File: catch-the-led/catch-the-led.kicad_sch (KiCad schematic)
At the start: 18 parts, among them SW1 SW_Push, U1 NE555P, U2 4017

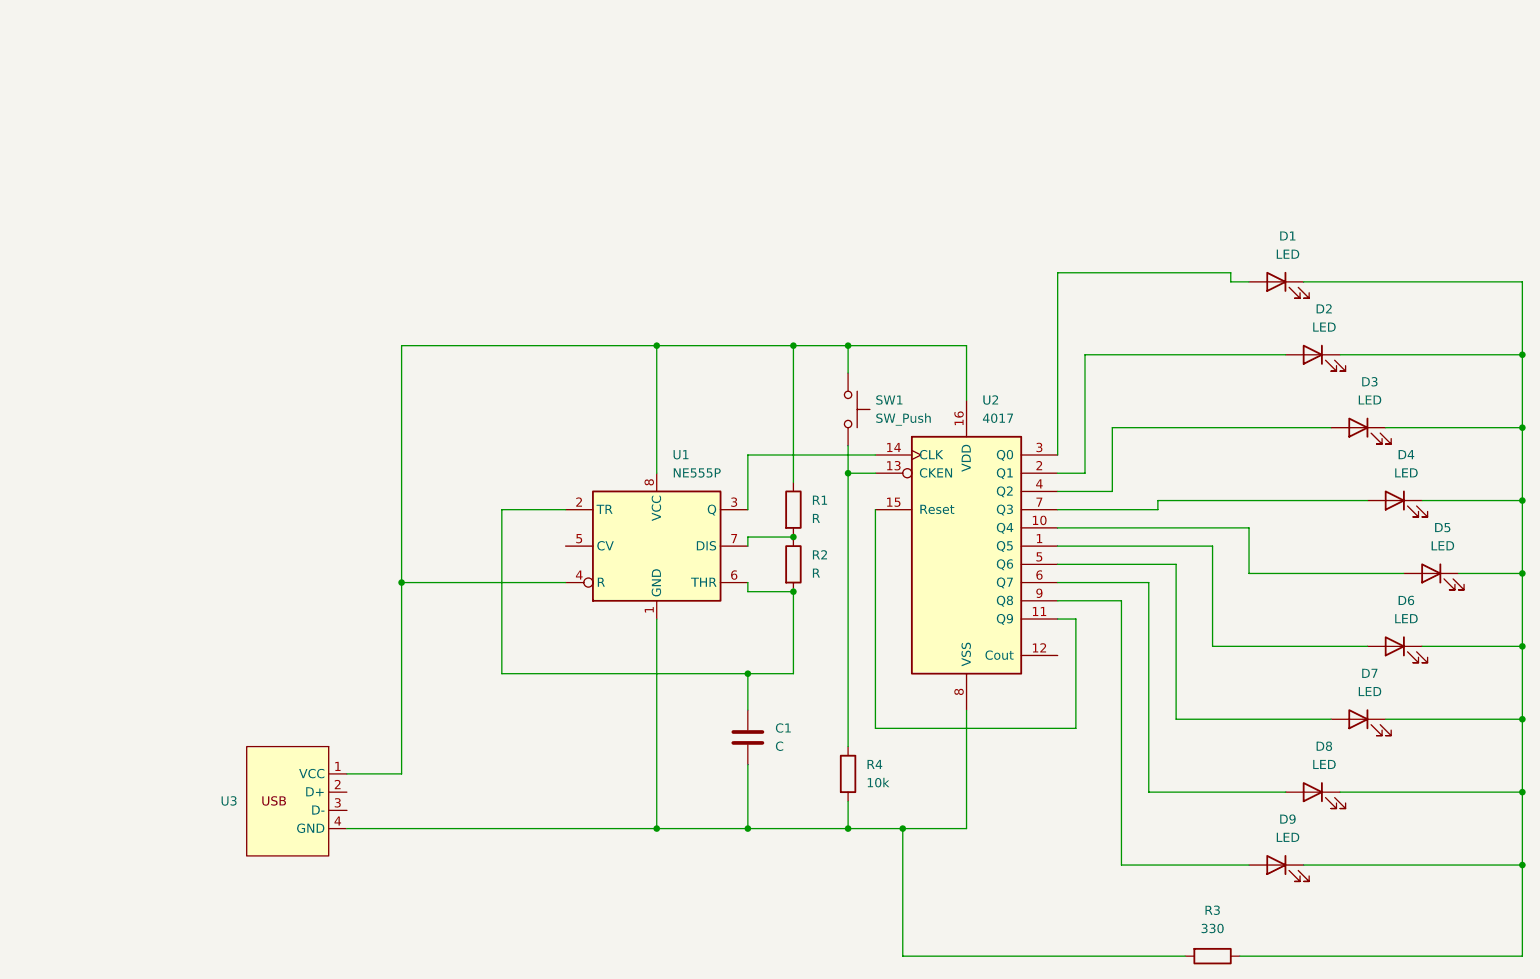
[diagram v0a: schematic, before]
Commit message: finished v2
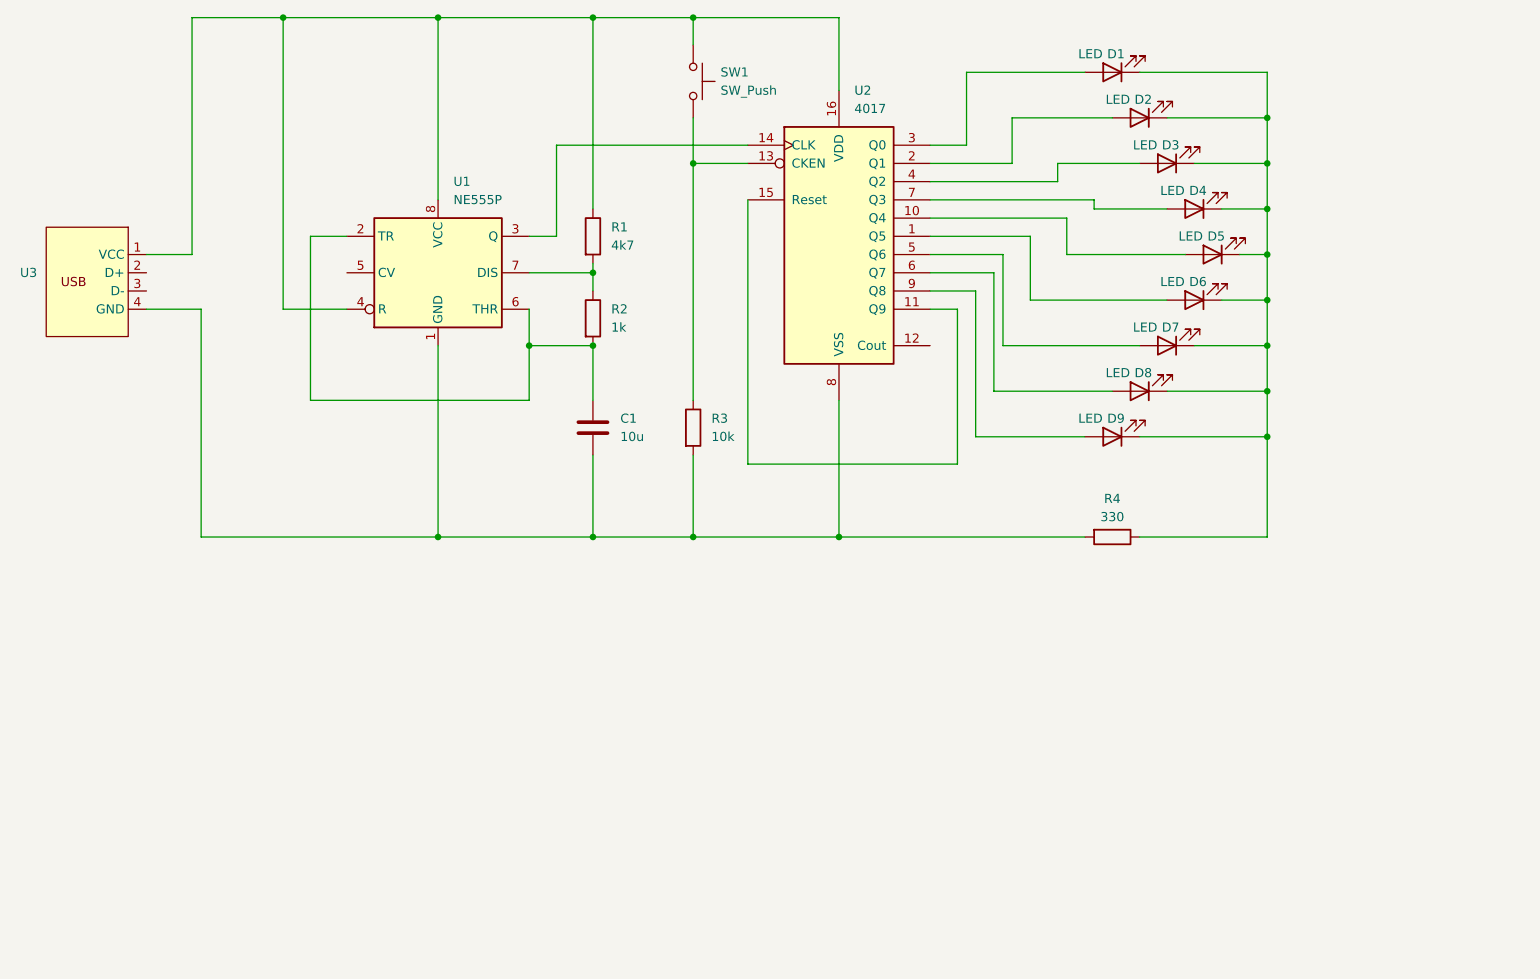
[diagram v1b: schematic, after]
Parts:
- C1: value C -> 10u
- R1: value R -> 4k7
- R2: value R -> 1k
- R3: value 330 -> 10k; footprint (none) -> Resistor_SMD:R_0805_2012Metric_Pad1.20x1.40mm_HandSolder
- R4: value 10k -> 330; footprint (none) -> Resistor_SMD:R_0805_2012Metric_Pad1.20x1.40mm_HandSolder
- SW1: footprint (none) -> Button_Switch_SMD:SW_SPST_TS-1088-xR020
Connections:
- net at D1.1 (K), D2.1 (K), D3.1 (K)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: now also R4.1; no longer R3.1
- net at SW1.2, U2.13 (CKEN): now also R3.1; no longer R4.1
